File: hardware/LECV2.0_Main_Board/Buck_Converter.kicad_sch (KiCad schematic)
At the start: 18 parts, among them U3 LMR33640ADDAR

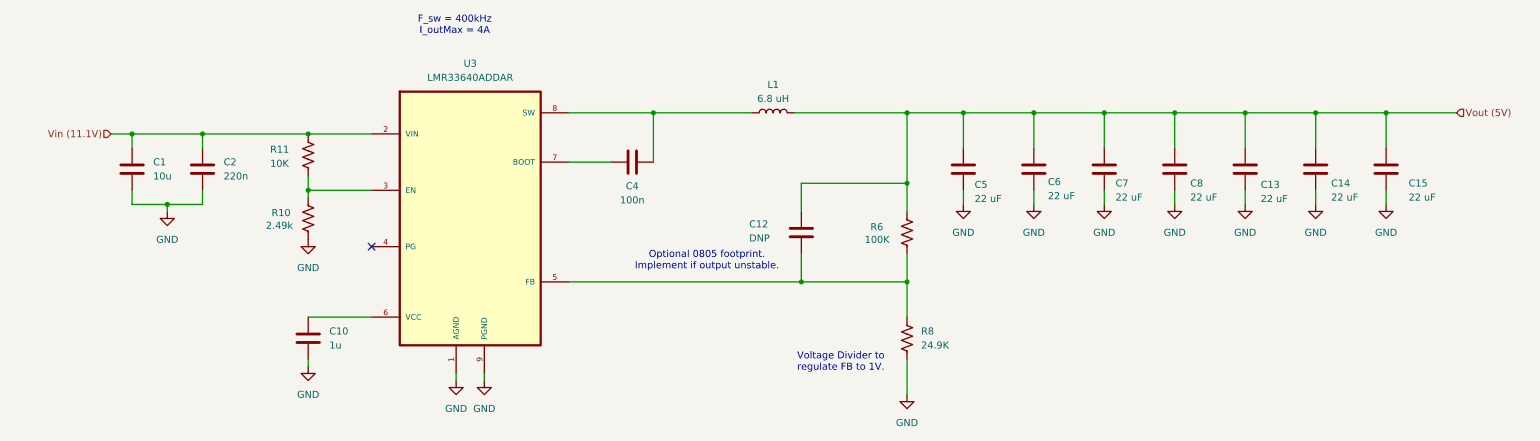
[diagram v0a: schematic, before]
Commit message: Finished PCBs
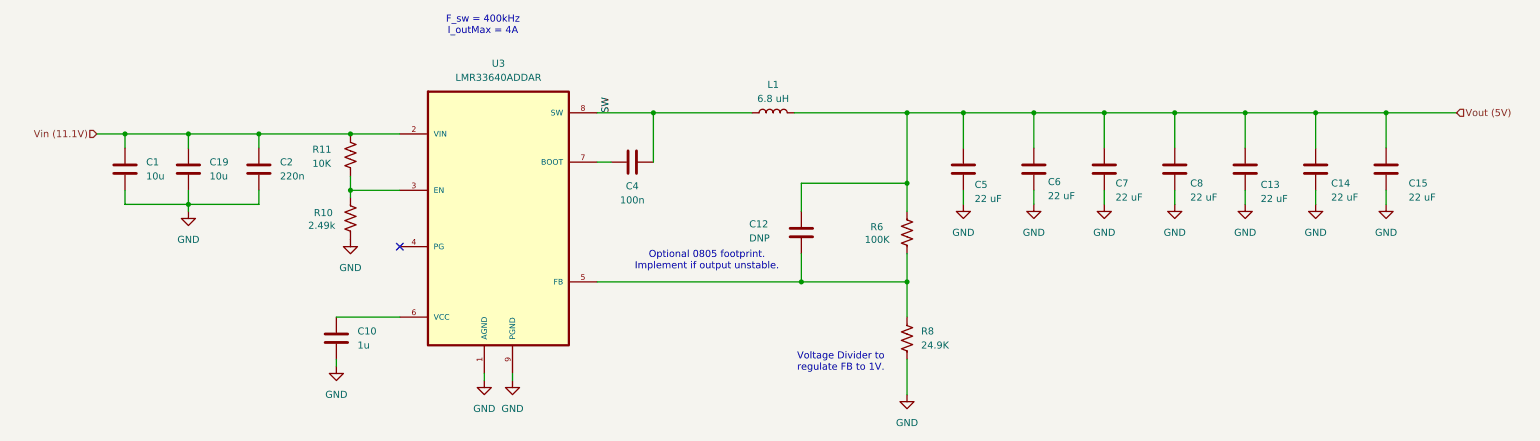
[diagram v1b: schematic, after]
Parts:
- added C19: 10u, Capacitor_SMD:C_1210_3225Metric, symbol Device:C
- C1: footprint Capacitor_SMD:C_0805_2012Metric -> Capacitor_SMD:C_1210_3225Metric; DigiKey https://www.digikey.com/en/products/detail/samsung-electro-mechanics/CL21A106KAYNNNE/3888549 -> https://www.digikey.com/en/products/detail/samsung-electro-mechanics/CL32B106KBJNNNE/3889045
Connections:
- net GND: now also C19.2
- net Vin (11.1V): now also C19.1
- net SW: now reaches C4.2, L1.1, U3.8 (SW)
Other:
- moved on the sheet: C1, C10, C2, R10, R11, U3
